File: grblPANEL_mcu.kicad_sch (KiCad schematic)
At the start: 31 parts, among them J201 2x5x1.27mm, J202 USB_C_Receptacle_USB2.0, SW201 SW_Push, SW202 SW_Push, U201 STM32G0B1CxTxN, U202 USBLC6-2SC6, Y201 8MHz

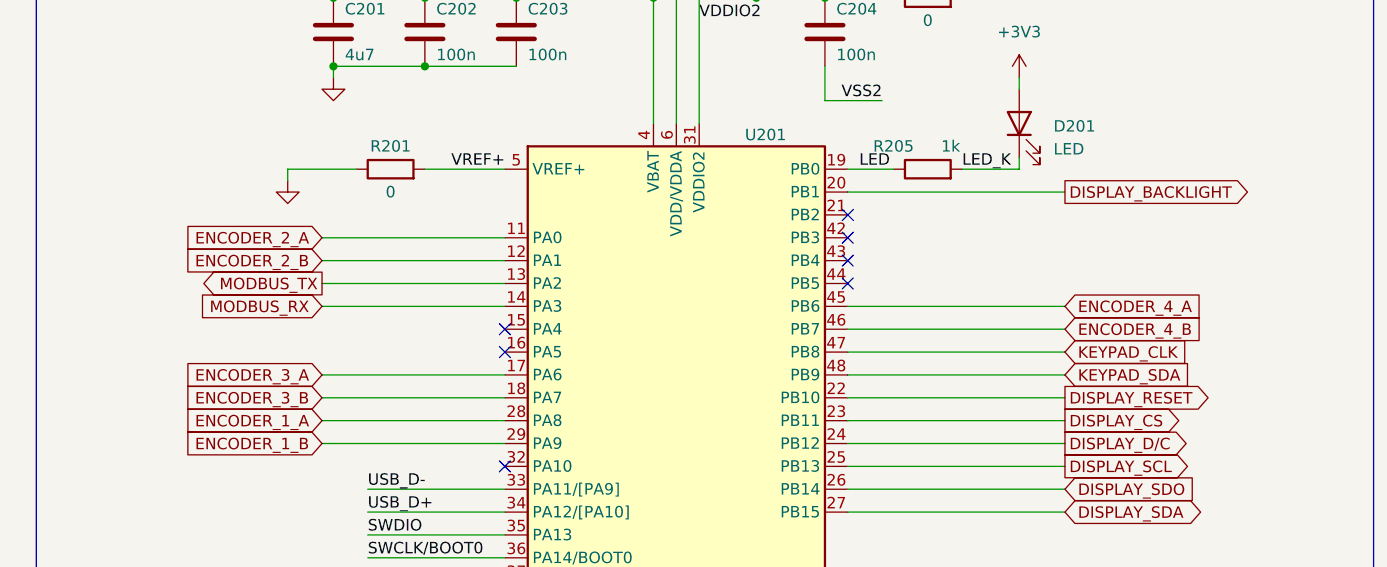
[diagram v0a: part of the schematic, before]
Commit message: more routing
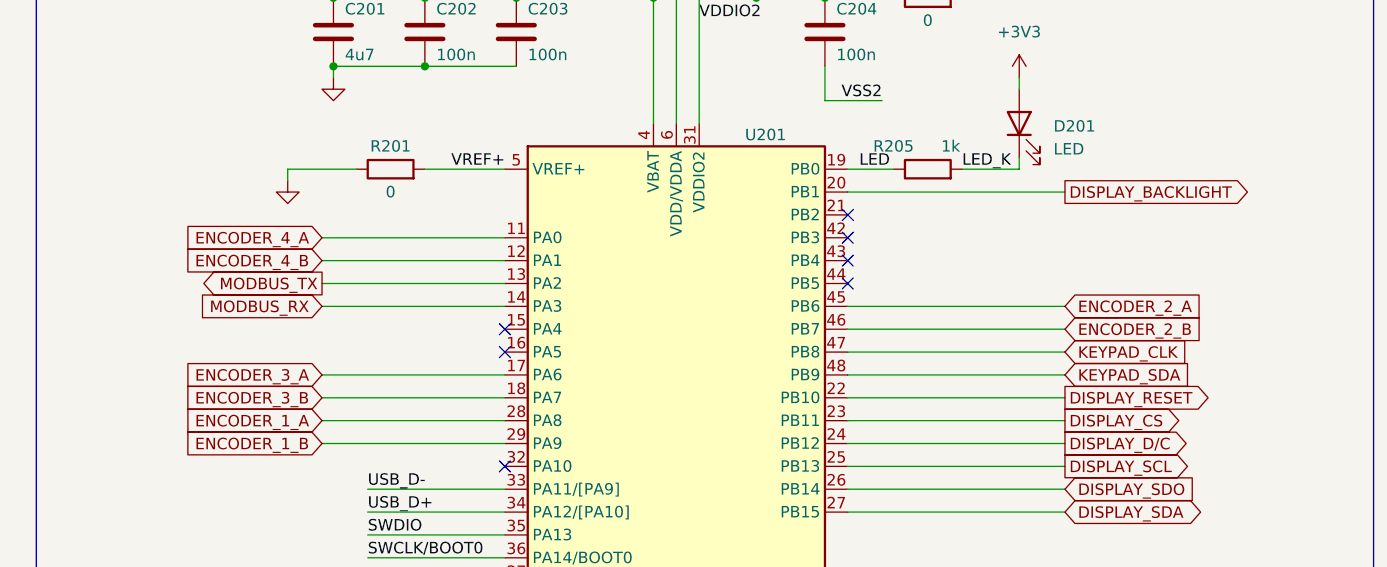
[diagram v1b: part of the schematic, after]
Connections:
- net ENCODER_2_A: now also U201.45 (PB6); no longer U201.11 (PA0)
- net ENCODER_2_B: now also U201.46 (PB7); no longer U201.12 (PA1)
- net ENCODER_4_A: now also U201.11 (PA0); no longer U201.45 (PB6)
- net ENCODER_4_B: now also U201.12 (PA1); no longer U201.46 (PB7)
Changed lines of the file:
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@@
     )
   )
-  (global_label "ENCODER_4_A" (shape input) (at 140.97 76.2 0) (fields_autoplaced)
+  (global_label "ENCODER_2_A" (shape input) (at 140.97 76.2 0) (fields_autoplaced)
     (effects (font (size 1.27 1.27)) (justify left))
     (property "Intersheet References" "${INTERSHEET_REFS}" (id 0) (at 156.3855 76.1206 0)
@@
     )
   )
-  (global_label "ENCODER_2_B" (shape input) (at 58.42 71.12 180) (fields_autoplaced)
+  (global_label "ENCODER_4_B" (shape input) (at 58.42 71.12 180) (fields_autoplaced)
     (effects (font (size 1.27 1.27)) (justify right))
     (property "Intersheet References" "${INTERSHEET_REFS}" (id 0) (at 42.8231 71.0406 0)
@@
     )
   )
-  (global_label "ENCODER_2_A" (shape input) (at 58.42 68.58 180) (fields_autoplaced)
+  (global_label "ENCODER_4_A" (shape input) (at 58.42 68.58 180) (fields_autoplaced)
     (effects (font (size 1.27 1.27)) (justify right))
     (property "Intersheet References" "${INTERSHEET_REFS}" (id 0) (at 43.0045 68.5006 0)
@@
     )
   )
-  (global_label "ENCODER_4_B" (shape input) (at 140.97 78.74 0) (fields_autoplaced)
+  (global_label "ENCODER_2_B" (shape input) (at 140.97 78.74 0) (fields_autoplaced)
     (effects (font (size 1.27 1.27)) (justify left))
     (property "Intersheet References" "${INTERSHEET_REFS}" (id 0) (at 156.5669 78.6606 0)
